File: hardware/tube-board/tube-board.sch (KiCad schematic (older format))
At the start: 18 parts, among them J1 CONN_01X10, J2 CONN_01X10, U1 HV5522PG, U2 HV5522PG

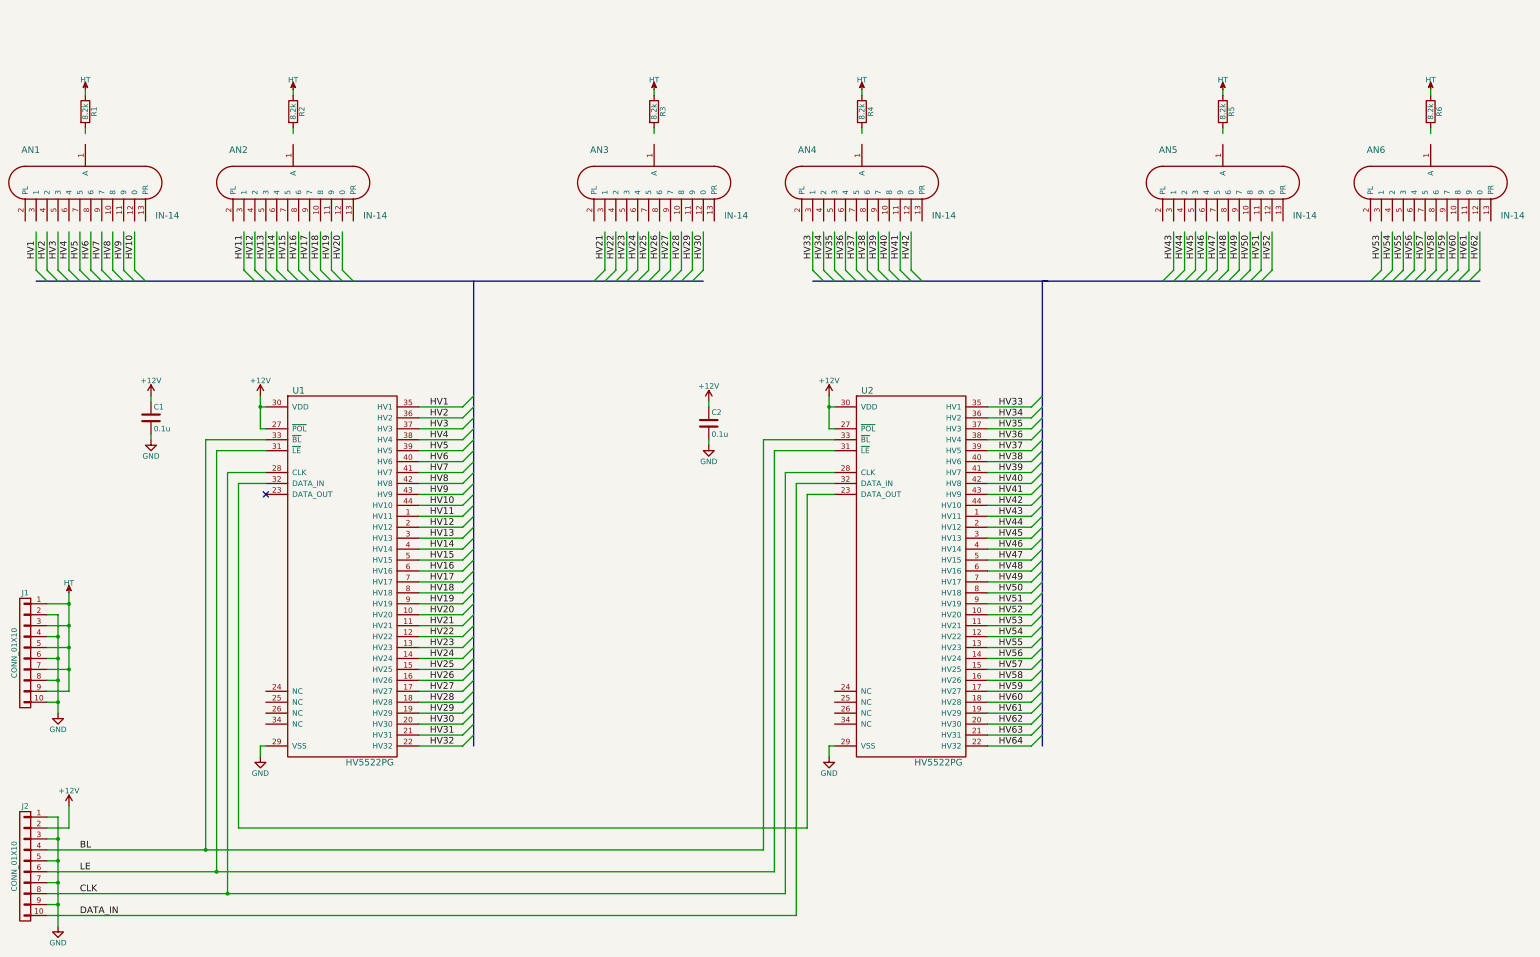
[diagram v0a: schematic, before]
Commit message: Working on footprints
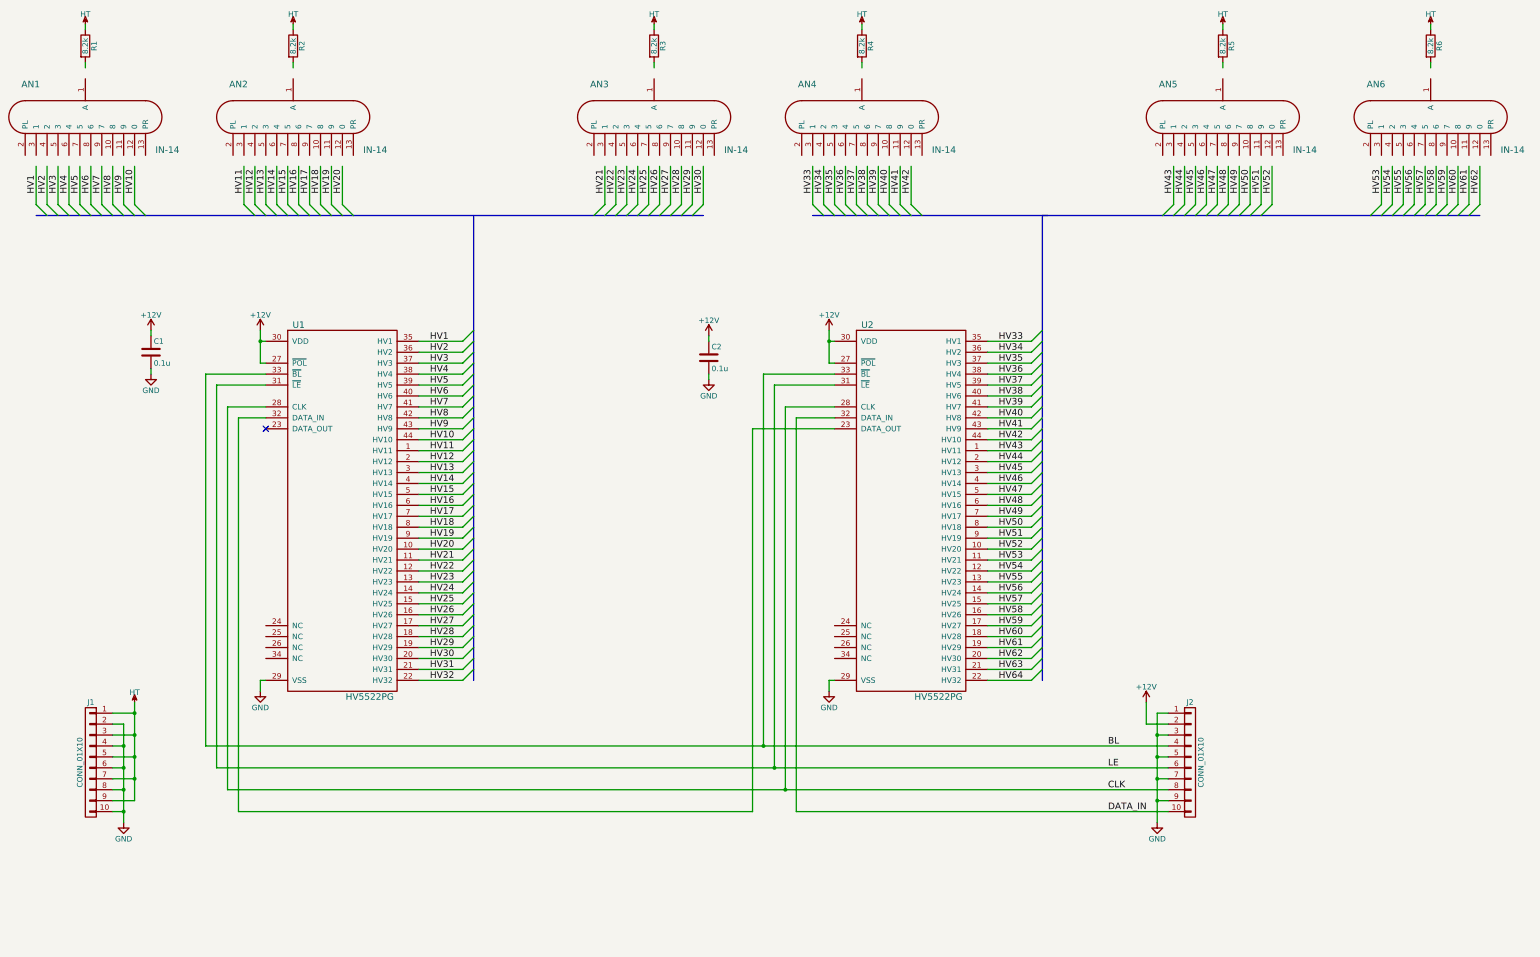
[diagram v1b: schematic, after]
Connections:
- wire segments 193 -> 210
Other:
- moved on the sheet: AN1, AN2, AN3, AN4, AN5, AN6, C1, C2, J1, J2, R1, R2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
